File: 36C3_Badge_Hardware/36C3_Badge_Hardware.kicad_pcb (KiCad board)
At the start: 2 copper layers, 160 x 100 mm, 0 parts

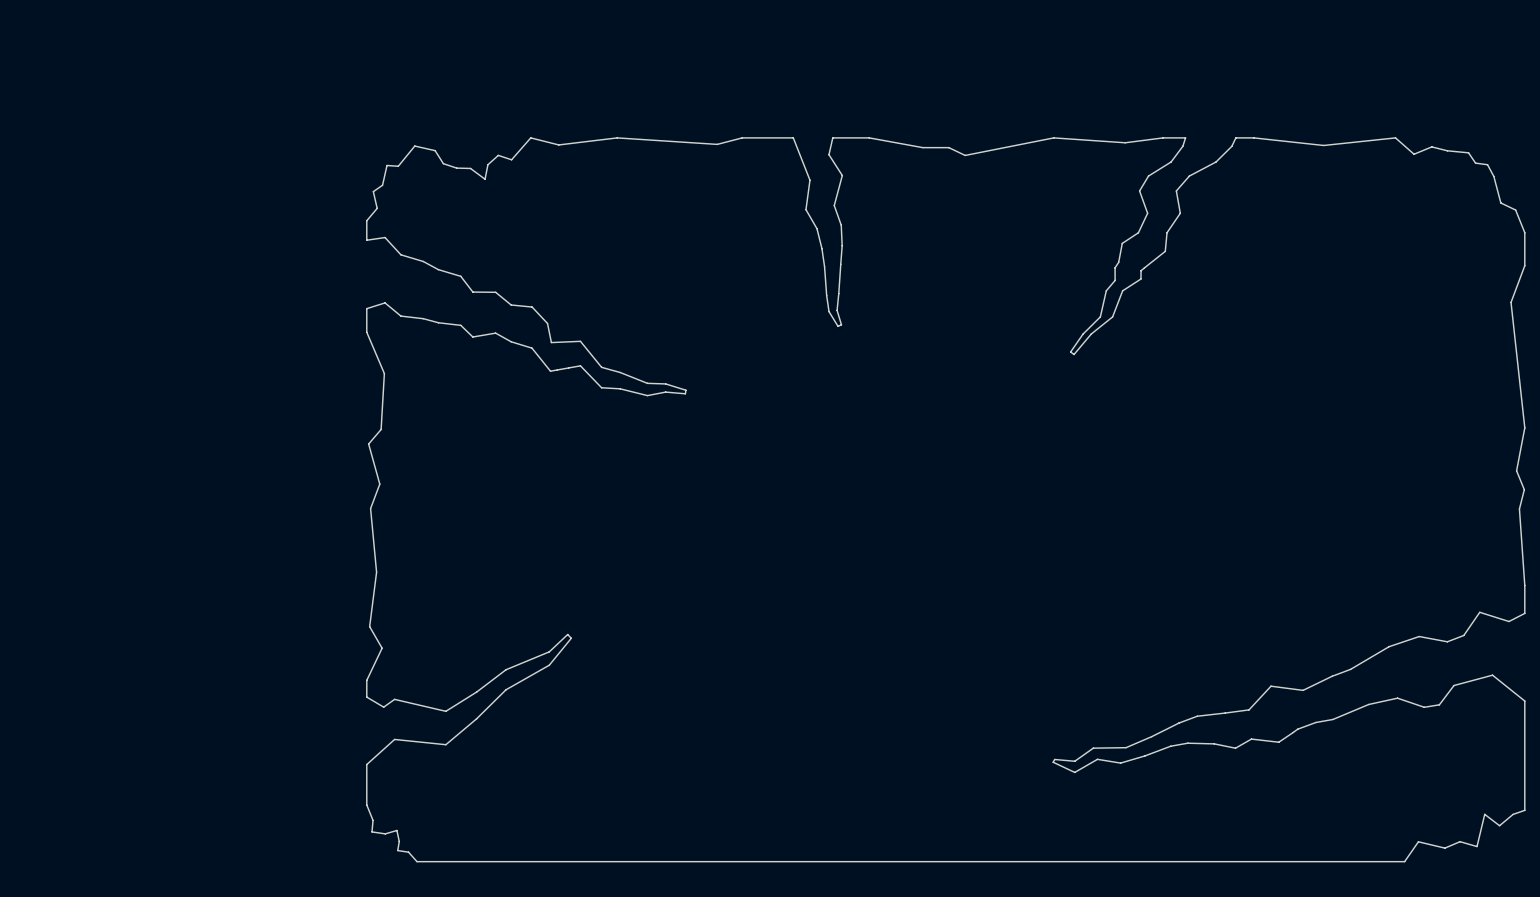
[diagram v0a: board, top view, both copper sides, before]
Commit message: First revision of PCB
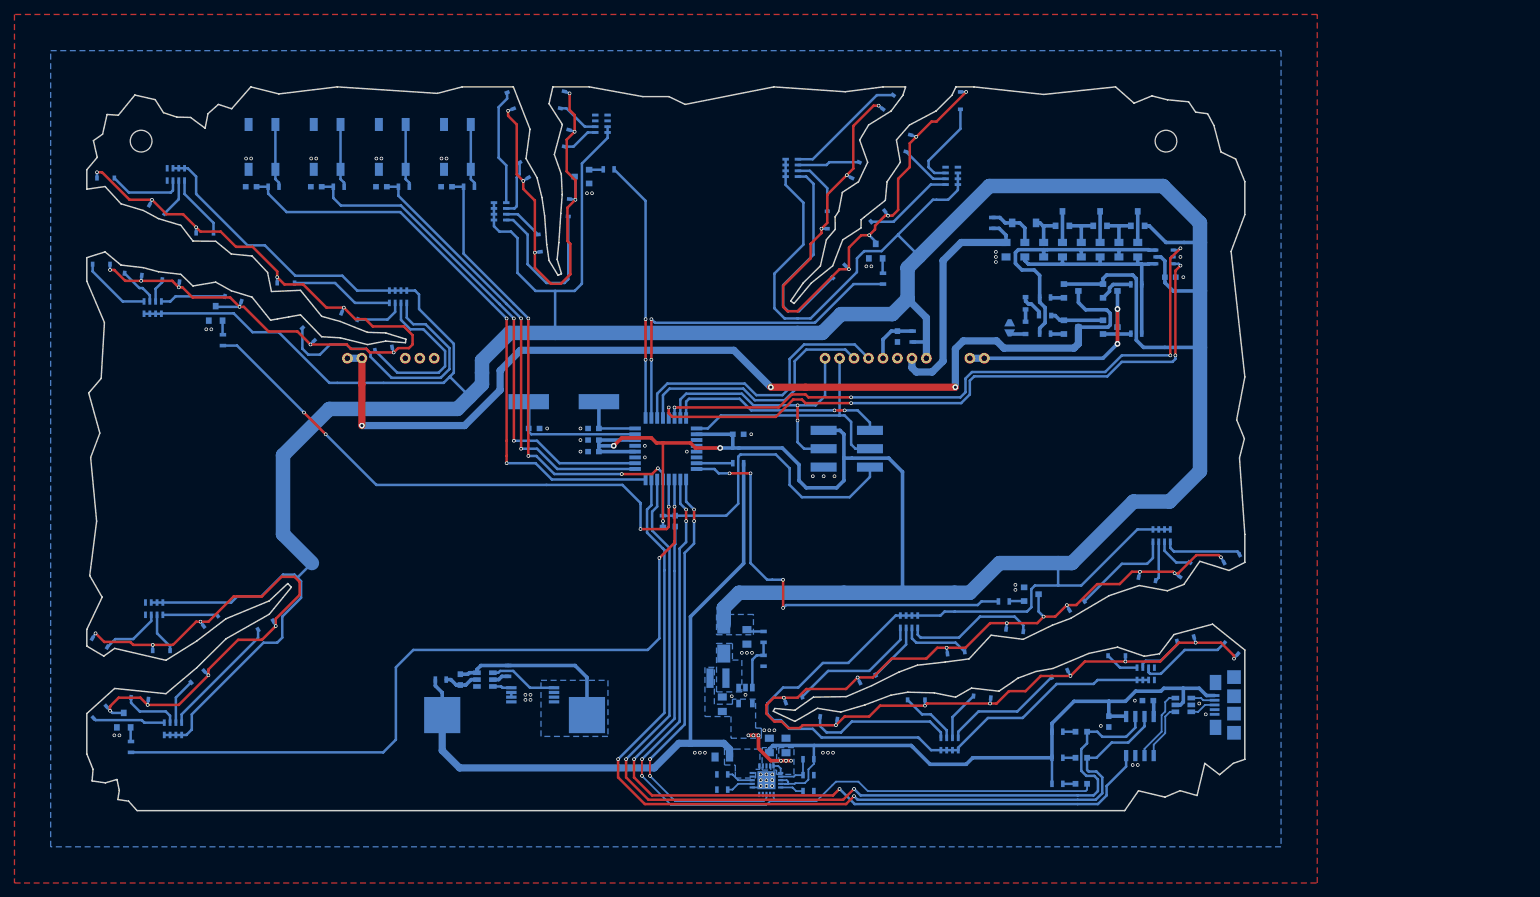
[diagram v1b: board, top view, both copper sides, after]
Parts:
- added BT1: 1S LiIon, custom:1S_18650_Holder_with_Spacers, B.Cu at (89.1, 116.8)
- added C1: 10µ/25V, Capacitors_SMD:C_0805, B.Cu at (124.3, 121.0)
- added C10: 470n/50V, Capacitors_SMD:C_0805, B.Cu at (175.2, 52.5)
- added C11: 470n/50V, Capacitors_SMD:C_0805, B.Cu at (172.6, 52.5)
- added C12: 470n/50V, Capacitors_SMD:C_0805, B.Cu at (170.0, 52.5)
- added C13: 470n/50V, Capacitors_SMD:C_0805, B.Cu at (167.4, 52.5)
- added C14: 470n/50V, Capacitors_SMD:C_0805, B.Cu at (164.8, 52.5)
- added C15: 470n/50V, Capacitors_SMD:C_0805, B.Cu at (162.2, 52.5)
- added C16: 470n/50V, Capacitors_SMD:C_0805, B.Cu at (159.6, 52.5)
- added C17: 470n/50V, Capacitors_SMD:C_0805, B.Cu at (157.0, 52.5)
- added C18: 100n, Capacitors_SMD:C_0603, B.Cu at (100.0, 80.4)
- added C19: 100n, Capacitors_SMD:C_0603, B.Cu at (100.0, 78.8)
- added C2: 4.7µ/25V, Capacitors_SMD:C_0805, B.Cu at (117.8, 115.3)
- added C20: 100n, Capacitors_SMD:C_0603, B.Cu at (120.0, 78.0)
- added C21: 100n, Capacitors_SMD:C_0603, B.Cu at (79.7, 43.8)
- added C22: 100n, Capacitors_SMD:C_0603, B.Cu at (70.7, 43.8)
- added C23: 82p, Capacitors_SMD:C_0603, B.Cu at (142.0, 64.5)
- added C24: 100n, Capacitors_SMD:C_0603, B.Cu at (61.7, 43.8)
- added C25: 100n, Capacitors_SMD:C_0603, B.Cu at (52.7, 43.8)
- added C26: 18p, Capacitors_SMD:C_0603, B.Cu at (100.0, 77.2)
- added C27: 100n, Capacitors_SMD:C_0603, B.Cu at (111.3, 90.0)
- added C28: 18p, Capacitors_SMD:C_0603, B.Cu at (91.8, 77.2)
- added C3: 100n, Capacitors_SMD:C_0603, B.Cu at (81.6, 111.9)
- added C4: 100n, Capacitors_SMD:C_0603, B.Cu at (171.2, 117.7)
- added C5: 100n, Capacitors_SMD:C_0603, B.Cu at (176.6, 114.8)
- added C6: 22µ/25V, Capacitors_SMD:C_0805, B.Cu at (121.2, 106.0)
- added C7: 4.7µ/25V, Capacitors_SMD:C_0805, B.Cu at (126.6, 121.0)
- added C8: 4.7µ/25V, Capacitors_SMD:C_0805, B.Cu at (117.8, 122.6)
- added C9: 100n, Capacitors_SMD:C_0603, B.Cu at (179.7, 56.3)
- added D1: USBLC6-2SC6, TO_SOT_Packages_SMD:SOT-23-6, B.Cu at (181.5, 115.4)
- added D10: Destruction3, custom:LED_SideFacing_0802, B.Cu at (133.9, 55.5)
- added D11: Destruction3, custom:LED_SideFacing_0802, B.Cu at (139.3, 47.9)
- added D12: Destruction3, custom:LED_SideFacing_0802, B.Cu at (143.5, 37.8)
- added D13: Destruction3, custom:LED_SideFacing_0802, B.Cu at (150.7, 31.9)
- added D14: Destruction2, custom:LED_SideFacing_0802, B.Cu at (32.0, 54.5)
- added D15: Destruction2, custom:LED_SideFacing_0802, B.Cu at (36.4, 55.9)
- added D16: Destruction2, custom:LED_SideFacing_0802, B.Cu at (41.6, 56.8)
- added D17: Destruction2, custom:LED_SideFacing_0802, B.Cu at (50.2, 59.3)
- added D18: Destruction2, custom:LED_SideFacing_0802, B.Cu at (60.6, 64.2)
- added D19: Destruction2, custom:LED_SideFacing_0802, B.Cu at (71.0, 66.2)
- added D2: SK110, Diodes_SMD:D_SMA_Standard, B.Cu at (118.0, 106.3)
- added D20: Destruction2, custom:LED_SideFacing_0802, B.Cu at (66.3, 61.7)
- added D21: Destruction2, custom:LED_SideFacing_0802, B.Cu at (57.5, 57.1)
- added D22: Destruction2, custom:LED_SideFacing_0802, B.Cu at (46.3, 50.2)
- added D23: Destruction2, custom:LED_SideFacing_0802, B.Cu at (39.7, 46.9)
- added D24: Destruction2, custom:LED_SideFacing_0802, B.Cu at (32.6, 42.6)
- added D25: Destruction1, custom:LED_SideFacing_0802, B.Cu at (31.8, 116.4)
- added D26: Destruction1, custom:LED_SideFacing_0802, B.Cu at (37.3, 114.5)
- added D27: Destruction1, custom:LED_SideFacing_0802, B.Cu at (45.3, 111.5)
- added D28: Destruction1, custom:LED_SideFacing_0802, B.Cu at (54.7, 104.4)
- added D29: Destruction1, custom:LED_SideFacing_0802, B.Cu at (47.1, 103.8)
- added D3: USB, LEDs:LED_0603, B.Cu at (167.4, 126.3)
- added D30: Destruction1, custom:LED_SideFacing_0802, B.Cu at (40.3, 107.9)
- added D31: Destruction1, custom:LED_SideFacing_0802, B.Cu at (31.8, 106.8)
- added D32: BAT54S, TO_SOT_Packages_SMD:SOT-23, B.Cu at (175.2, 48.2)
- added D33: BAT54S, TO_SOT_Packages_SMD:SOT-23, B.Cu at (170.0, 48.2)
- added D34: Hope2, custom:LED_SideFacing_0802, B.Cu at (188.2, 95.2)
- added D35: Hope2, custom:LED_SideFacing_0802, B.Cu at (181.7, 96.7)
- added D36: Hope2, custom:LED_SideFacing_0802, B.Cu at (176.5, 98.0)
- added D37: Hope2, custom:LED_SideFacing_0802, B.Cu at (166.8, 101.7)
- added D38: Hope2, custom:LED_SideFacing_0802, B.Cu at (158.2, 105.1)
- added D39: Hope2, custom:LED_SideFacing_0802, B.Cu at (150.1, 108.2)
- added D4: Rx, LEDs:LED_0603, B.Cu at (167.4, 122.7)
- added D40: Hope2, custom:LED_SideFacing_0802, B.Cu at (137.9, 111.8)
- added D41: Hope2, custom:LED_SideFacing_0802, B.Cu at (127.7, 114.7)
- added D42: Hope2, custom:LED_SideFacing_0802, B.Cu at (132.5, 117.2)
- added D43: Hope2, custom:LED_SideFacing_0802, B.Cu at (144.6, 114.7)
- added D44: Hope2, custom:LED_SideFacing_0802, B.Cu at (153.7, 114.3)
- added D45: Hope2, custom:LED_SideFacing_0802, B.Cu at (164.4, 111.1)
- added D46: Hope2, custom:LED_SideFacing_0802, B.Cu at (172.3, 108.6)
- added D47: Hope2, custom:LED_SideFacing_0802, B.Cu at (181.8, 106.3)
- added D48: Hope2, custom:LED_SideFacing_0802, B.Cu at (188.1, 107.6)
- added D49: BAT54S, TO_SOT_Packages_SMD:SOT-23, B.Cu at (164.8, 48.2)
- added D5: Tx, LEDs:LED_0603, B.Cu at (167.4, 119.1)
- added D50: Hope1, custom:LED_SideFacing_0802, B.Cu at (88.5, 31.9)
- added D51: Hope1, custom:LED_SideFacing_0802, B.Cu at (90.4, 41.5)
- added D52: Hope1, custom:LED_SideFacing_0802, B.Cu at (92.5, 51.6)
- added D53: Hope1, custom:LED_SideFacing_0802, B.Cu at (96.6, 46.7)
- added D54: Hope1, custom:LED_SideFacing_0802, B.Cu at (96.3, 37.1)
- added D55: Hope1, custom:LED_SideFacing_0802, B.Cu at (95.7, 31.8)
- added D56: BAT46W, Diodes_SMD:D_SOD-123, B.Cu at (159.5, 48.8)
- added D57: 1N4148, Diodes_SMD:D_0603, B.Cu at (162.4, 61.6)
- added D58: 1N4148, Diodes_SMD:D_0603, B.Cu at (159.7, 59.9)
- added D59: 1N4148, Diodes_SMD:D_0603, B.Cu at (159.7, 63.3)
- added D7: Destruction3, custom:LED_SideFacing_0802, B.Cu at (140.7, 32.1)
- added D8: Destruction3, custom:LED_SideFacing_0802, B.Cu at (136.2, 41.5)
- added D9: Destruction3, custom:LED_SideFacing_0802, B.Cu at (132.3, 48.4)
- added G***: resource_exhaustion_mask, custom:resource_exhaustion_mask, F.Cu at (84.1, 103.3)
- added J1: MicroUSB, custom:MicroUSB_Amphenol_10118192, B.Cu at (188.5, 115.4)
- added J2: ISP, Pin_Headers:Pin_Header_Straight_SMT_02x03, B.Cu at (135.0, 80.0)
- added JP1: ISP, custom:Jumper_SolderBridge, B.Cu at (157.5, 63.3)
- added L1: 4.7µ/1.25A, custom:Inductor_3x3mm, B.Cu at (117.2, 111.7)
- added Q1: FS8205A, Housings_SSOP:TSSOP-8_4.4x3mm_Pitch0.65mm, B.Cu at (91.6, 114.0)
- added Q10: MMBTA42, TO_SOT_Packages_SMD:SOT-23, B.Cu at (98.4, 42.4)
- added Q2: MMBTA42, TO_SOT_Packages_SMD:SOT-23, B.Cu at (139.0, 52.7)
- added Q3: MMBTA42, TO_SOT_Packages_SMD:SOT-23, B.Cu at (47.8, 61.3)
- added Q4: MMBTA92, TO_SOT_Packages_SMD:SOT-23, B.Cu at (171.4, 58.2)
- added Q5: MMBTA42, TO_SOT_Packages_SMD:SOT-23, B.Cu at (171.4, 63.2)
- added Q6: MMBTA42, TO_SOT_Packages_SMD:SOT-23, B.Cu at (35.1, 117.5)
- added Q7: MMBTA42, TO_SOT_Packages_SMD:SOT-23, B.Cu at (160.5, 100.1)
- added Q8: MMBTA92, TO_SOT_Packages_SMD:SOT-23, B.Cu at (166.0, 58.2)
- added Q9: MMBTA42, TO_SOT_Packages_SMD:SOT-23, B.Cu at (166.0, 63.2)
- added R1: 100R, Resistors_SMD:R_0603, B.Cu at (78.9, 111.9)
- added R10: 1k, Resistors_SMD:R_0603, B.Cu at (164.1, 126.3)
- added R11: 1k, Resistors_SMD:R_0603, B.Cu at (164.1, 122.7)
- added R12: 1k, Resistors_SMD:R_0603, B.Cu at (164.1, 119.1)
- added R14: 1k, Resistors_SMD:R_Array_Concave_4x0603, B.Cu at (127.4, 41.2)
- added R15: 1k, Resistors_SMD:R_Array_Concave_4x0603, B.Cu at (149.5, 42.3)
- added R16: 4.7k, Resistors_SMD:R_0603, B.Cu at (140.0, 56.5)
- added R17: 1k, Resistors_SMD:R_Array_Concave_4x0603, B.Cu at (39.1, 60.5)
- added R18: 1k, Resistors_SMD:R_Array_Concave_4x0603, B.Cu at (73.0, 59.0)
- added R19: 1k, Resistors_SMD:R_Array_Concave_4x0603, B.Cu at (42.3, 42.1)
- added R2: 2k, Resistors_SMD:R_0603, B.Cu at (117.8, 125.0)
- added R20: 4.7k, Resistors_SMD:R_0603, B.Cu at (48.8, 65.0)
- added R21: 1k, Resistors_SMD:R_0603, B.Cu at (175.0, 57.3)
- added R22: 1k, Resistors_SMD:R_0603, B.Cu at (175.0, 64.1)
- added R23: 1k, Resistors_SMD:R_Array_Concave_4x0603, B.Cu at (41.9, 118.7)
- added R24: 1k, Resistors_SMD:R_Array_Concave_4x0603, B.Cu at (39.3, 102.1)
- added R25: 4.7k, Resistors_SMD:R_0603, B.Cu at (36.1, 121.2)
- added R26: 1k, Resistors_SMD:R_Array_Concave_4x0603, B.Cu at (178.5, 92.0)
- added R27: 1k, Resistors_SMD:R_Array_Concave_4x0603, B.Cu at (143.6, 103.9)
- added R28: 1k, Resistors_SMD:R_Array_Concave_4x0603, B.Cu at (149.2, 120.8)
- added R29: 1k, Resistors_SMD:R_Array_Concave_4x0603, B.Cu at (176.3, 111.1)
- added R3: 1k, Resistors_SMD:R_0603, B.Cu at (88.2, 110.7)
- added R30: 4.7k, Resistors_SMD:R_0603, B.Cu at (156.7, 101.1)
- added R31: 1k, Resistors_SMD:R_0603, B.Cu at (162.4, 59.1)
- added R32: 1k, Resistors_SMD:R_0603, B.Cu at (162.4, 64.1)
- added R33: 1k, Resistors_SMD:R_Array_Concave_4x0603, B.Cu at (87.1, 47.2)
- added R34: 1k, Resistors_SMD:R_Array_Concave_4x0603, B.Cu at (101.1, 35.1)
- added R35: 470R, Resistors_SMD:R_0603, B.Cu at (155.1, 48.8)
- added R36: 4.7k, Resistors_SMD:R_0603, B.Cu at (102.1, 41.4)
- added R37: 1k, Resistors_SMD:R_0603, B.Cu at (82.8, 43.8)
- added R38: 1k, Resistors_SMD:R_0603, B.Cu at (73.8, 43.8)
- added R39: 8.2k, Resistors_SMD:R_0603, B.Cu at (144.1, 64.5)
- added R4: 330k, Resistors_SMD:R_0603, B.Cu at (129.7, 122.9)
- added R40: 1k, Resistors_SMD:R_0603, B.Cu at (64.8, 43.8)
- added R41: 1k, Resistors_SMD:R_0603, B.Cu at (55.8, 43.8)
- added R42: 100k, Resistors_SMD:R_0603, B.Cu at (120.0, 82.0)
- added R43: 10k, Resistors_SMD:R_0603, B.Cu at (109.6, 90.0)
- added R5: 120k, Resistors_SMD:R_0603, B.Cu at (129.7, 125.1)
- added R6: 18k, Resistors_SMD:R_0603, B.Cu at (117.8, 127.1)
- added R7: 10k, Resistors_SMD:R_0603, B.Cu at (129.7, 127.3)
- added R8: 5.6k, Resistors_SMD:R_0603, B.Cu at (123.5, 106.0)
- added R9: 1.82k, Resistors_SMD:R_0603, B.Cu at (123.5, 109.3)
- added REF**: MountingHole_3mm, Mounting_Holes:MountingHole_3mm, F.Cu at (179.1, 37.5)
- added REF**: StandBy_H3.5mm, custom:StandBy_H3.5mm, B.Cu at (54.2, 49.6)
- added REF**: MountingHole_3mm, Mounting_Holes:MountingHole_3mm, F.Cu at (37.5, 37.5)
- added SW1: Reset, Buttons_Switches_SMD:SW_SPST_SKQG, B.Cu at (81.2, 38.3)
- added SW2: Button1, Buttons_Switches_SMD:SW_SPST_SKQG, B.Cu at (72.2, 38.3)
- added SW3: Button2, Buttons_Switches_SMD:SW_SPST_SKQG, B.Cu at (63.2, 38.3)
- added SW4: Standby, Buttons_Switches_SMD:SW_SPST_SKQG, B.Cu at (54.2, 38.3)
- added U1: MIC2288, TO_SOT_Packages_SMD:SOT-23-5, B.Cu at (121.0, 114.1)
- added U2: DW01, TO_SOT_Packages_SMD:SOT-23-6, B.Cu at (85.0, 111.9)
- added U3: MCP73871-2CCI, Housings_DFN_QFN:QFN-20-1EP_4x4mm_Pitch0.5mm, B.Cu at (123.9, 125.8)
- added U4: CH330N, Housings_SOIC:SOIC-8_3.9x4.9mm_Pitch1.27mm, B.Cu at (175.5, 119.7)
- added U5: 74LVC2G17, custom:SOT-457, B.Cu at (178.9, 53.5)
- added U6: ATMEGA328P-AU, Housings_QFP:TQFP-32_7x7mm_Pitch0.8mm, B.Cu at (110.0, 80.0)
- added VFD1: HCS-12SS59T, custom:VFD_HCS-12SS59T_noSilk, F.Cu at (110.0, 80.0)
- added Y1: 16MHz, Crystals:Crystal_HC49-SD_SMD, B.Cu at (95.9, 73.5)
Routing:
- net +5V: track 0.00 -> 850.7 mm, vias 0 -> 3
- net Net-(D34-Pad1): track 0.00 -> 160.0 mm, vias 0 -> 16
- net /FIL+: track 0.00 -> 139.8 mm, vias 0 -> 3
- net /UART_RX: track 0.00 -> 132.0 mm, vias 0 -> 2
- net /UART_TX: track 0.00 -> 131.8 mm, vias 0 -> 2
- net Net-(D14-Pad1): track 0.00 -> 113.6 mm, vias 0 -> 11
- net /UART_RTS: track 0.00 -> 111.7 mm, vias 0 -> 2
- net /SW_RESET: track 0.00 -> 110.8 mm, vias 0 -> 4
- net /PMIC_~PG: track 0.00 -> 110.6 mm, vias 0 -> 4
- net /LED_D1: track 0.00 -> 108.2 mm, vias 0 -> 2
- net +BATT: track 0.00 -> 95.5 mm
- net +5V_USB: track 0.00 -> 92.7 mm
- net /VFD_SUP_CLK_A: track 0.00 -> 91.6 mm, vias 0 -> 4
- net /VFD_SUP_CLK_B: track 0.00 -> 90.9 mm, vias 0 -> 4
- net Net-(D10-Pad1): track 0.00 -> 85.4 mm, vias 0 -> 8
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- added copper zone on B.Cu, net +5V
- added copper zone on B.Cu, net +5V_USB
- added copper zone on B.Cu, net +BATT
- added copper zone on B.Cu, net -BATT
- added copper zone on B.Cu, net GND
- added copper zone on F.Cu, net GND
- added copper zone on B.Cu, net Net-(D2-Pad2)
- added copper zone on B.Cu, net VCC
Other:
- rule via_min_drill: 0.3 -> 0.2
- board text added: "A"
- board text added: "B"
- board text added: "Designed by Cato - @Mezgrman Rev. 1.0 / 08.12.2019"
- board text added: "I"
- board text added: "O"
- board text added: "Reset"
- board text added: "USB"
